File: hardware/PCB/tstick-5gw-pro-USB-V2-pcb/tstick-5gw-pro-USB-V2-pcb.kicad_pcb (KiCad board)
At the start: 4 copper layers, 55.9 x 25.4 mm, 62 parts, among them J1 USB_C_Receptacle_USB2.0, Q1 BSS138, Q2 BSS138, Q3 BSS138, SW1 JST-SH-1.00mm 1x2, SW2 PTS810 SJM Switch, SW3 PTS810 SJM Switch, U2 MCP73871, U3 NCP167AMX330TBG, U4 NCP167AMX180TBG

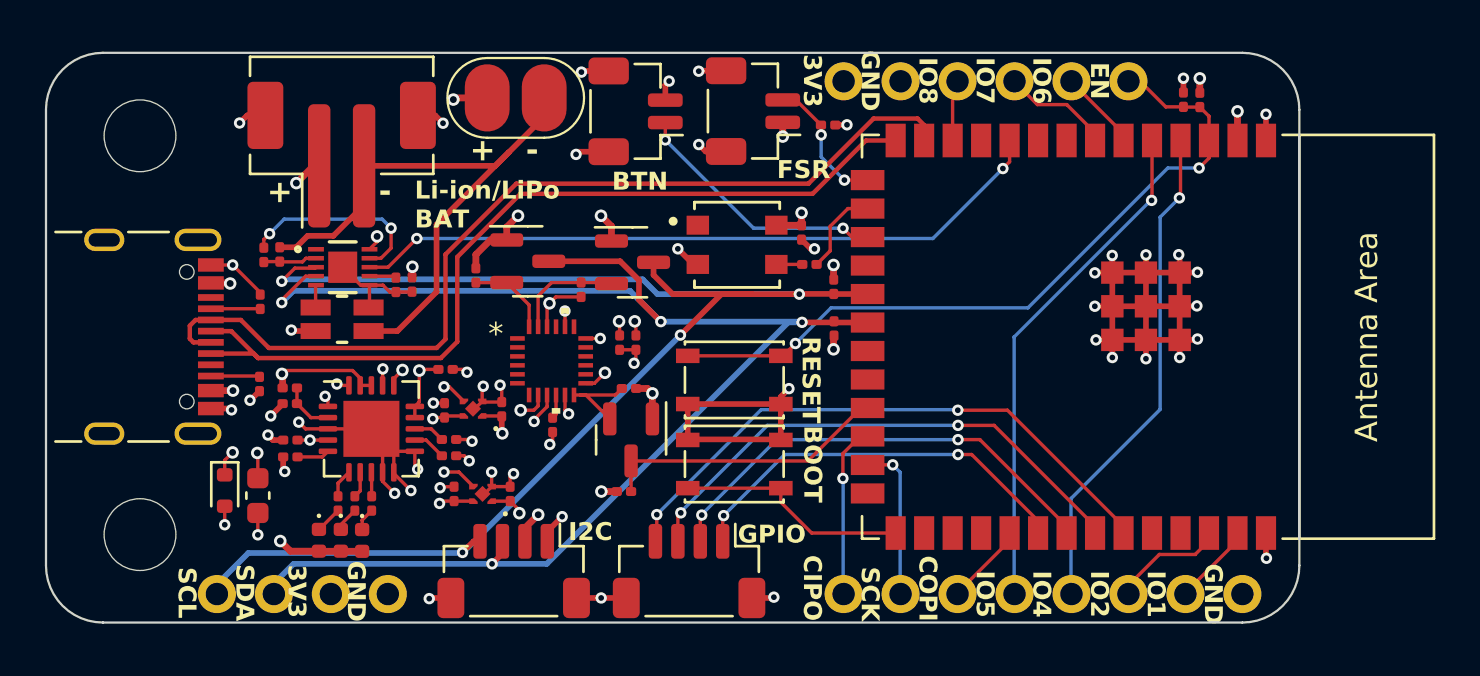
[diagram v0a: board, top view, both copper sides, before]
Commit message: added updated bill of materials and manufacturing files
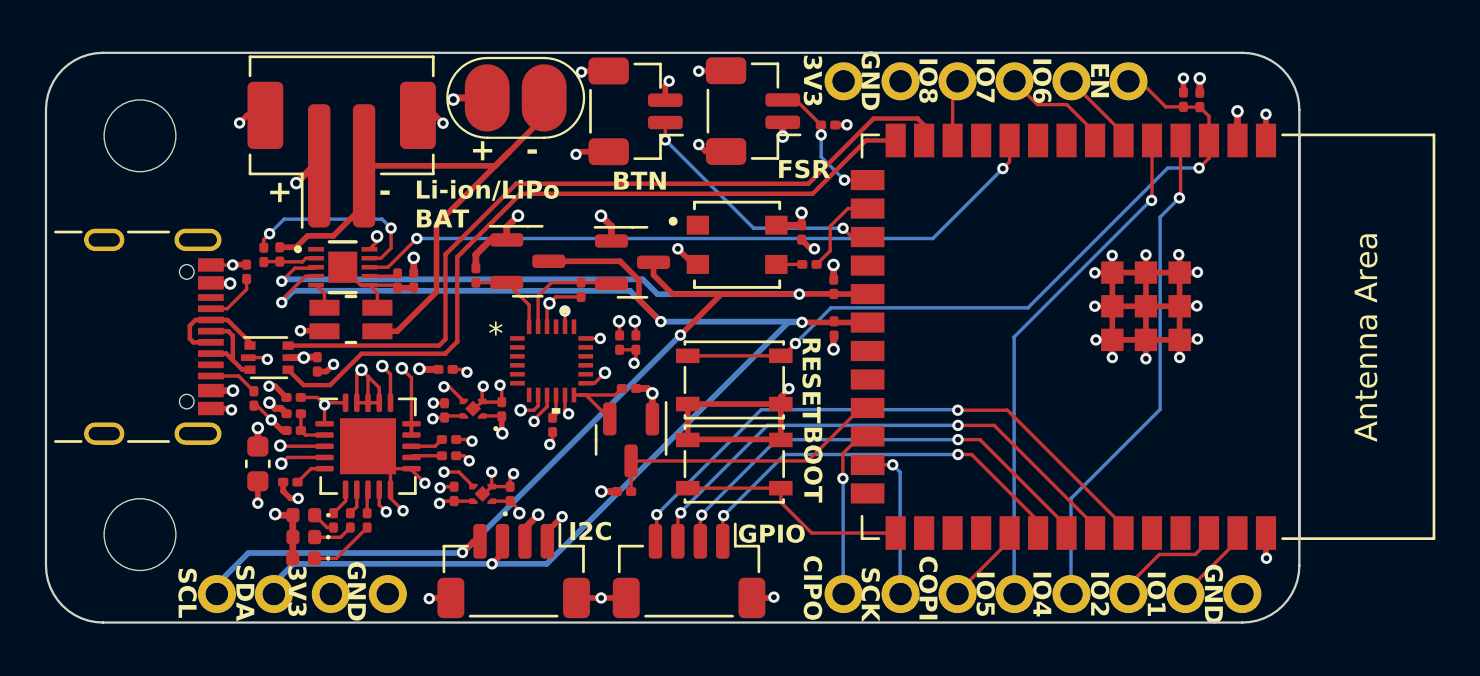
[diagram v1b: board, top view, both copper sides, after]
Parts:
- removed D2: ESD5Zxx, Diode_SMD:D_SOD-523
- added C15: 0.1uF, Capacitor_SMD:C_0201_0603Metric, F.Cu at (106.1, 62.1)
- added U1: USBLC6-2P6, Package_TO_SOT_SMD:SOT-666, F.Cu at (103.9, 61.9)
- TrillExtensionInput1: value JST-SH 1x08 1.00mm -> JST-SH-1x04 1.0mm
- moved CHARGLED1 2.73 mm to (105.5, 70.8), turned to 180 degrees
- moved C3 1.91 mm to (105.0, 63.6)
- moved CHARGLED2 1.66 mm to (105.5, 69.8), turned to 180 degrees
- moved R7 1.47 mm to (102.9, 58.0)
- moved C14 1.41 mm to (103.4, 66.6)
- moved CHARGLED3 1.31 mm to (105.5, 68.9), turned to 180 degrees
- moved R4 1.21 mm to (105.0, 65.1)
- moved R18 1.16 mm to (105.0, 64.3)
- moved TH2 1.12 mm to (104.9, 67.4)
- moved U2 0.79 mm to (108.3, 65.8)
- moved R22 0.78 mm to (107.5, 69.1)
- moved R24 0.78 mm to (106.8, 69.1)
- moved R3 0.78 mm to (108.3, 69.1)
- moved R6 0.69 mm to (103.2, 63.7)
- moved R2 0.39 mm to (107.6, 60.1)
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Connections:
- J1 pad A6: /USBD+ -> /D+
- J1 pad A7: /USBD- -> /D-
- J1 pad B6: /USBD+ -> /D+
- J1 pad B7: /USBD- -> /D-
- U2 pad 17: SYS -> VUSB
- U2 pad 3: GND -> VUSB
- U2 pad 4: SYS -> VUSB
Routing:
- net /USBD-: track 42.2 -> 35.6 mm
- net /USBD+: track 39.4 -> 34.1 mm
- net /D-: track 0.00 -> 4.93 mm
- net GND: track 95.5 -> 90.5 mm, vias 58 -> 57
- net /D+: track 0.00 -> 4.20 mm
- net VUSB: track 13.2 -> 17.2 mm, vias 6 -> 9
- net +BATT: track 7.97 -> 10.6 mm, vias 6 -> 7
- net Net-(CHARGLED1-K): track 1.02 -> 2.92 mm
- net Net-(CHARGLED2-K): track 1.10 -> 1.77 mm
- net SYS: track 8.89 -> 8.75 mm, vias 8 -> 5
